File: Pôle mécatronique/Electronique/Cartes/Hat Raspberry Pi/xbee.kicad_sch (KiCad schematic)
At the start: 1 part

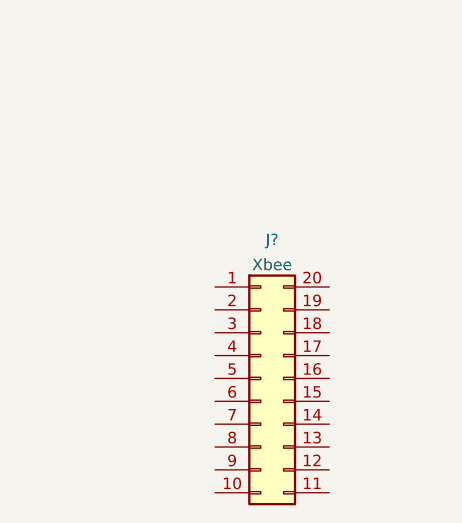
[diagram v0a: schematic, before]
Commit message: Reprise backup
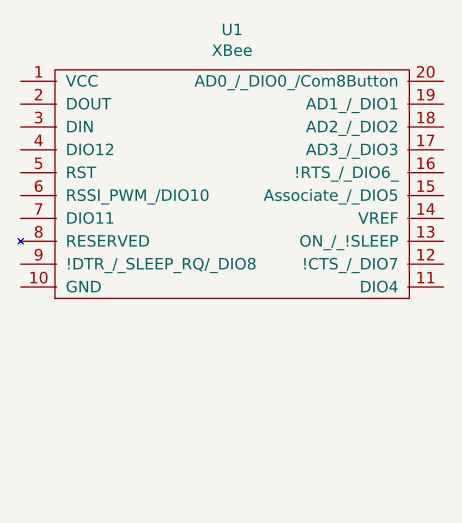
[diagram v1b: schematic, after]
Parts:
- removed J?: Xbee, symbol Connector_Generic:Conn_02x10_Counter_Clockwise
- added U1: XBee, Connecteurs:XBEE_PRO-20_THT, symbol bus_raspi-rescue:XBeePro-xbeepro
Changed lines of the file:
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@@
 (kicad_sch (version 20211123) (generator eeschema)
   (paper "A4")
-  (symbol (lib_id "Connector_Generic:Conn_02x10_Counter_Clockwise") (at 120.65 88.9 0) (unit 1)
-    (in_bom yes) (on_board yes) (fields_autoplaced)
-    (property "Reference" "J?" (id 0) (at 121.92 73.5035 0))
-    (property "Value" "Xbee" (id 1) (at 121.92 76.2786 0))
-    (property "Footprint" "" (id 2) (at 120.65 88.9 0)
+  (symbol (lib_id "bus_raspi-rescue:XBeePro-xbeepro") (at 93.98 85.09 0) (unit 1)
+    (in_bom yes) (on_board yes)
+    (property "Reference" "U1" (id 0) (at 117.475 50.165 0))
+    (property "Value" "XBee" (id 1) (at 117.475 52.4764 0))
+    (property "Footprint" "Connecteurs:XBEE_PRO-20_THT" (id 2) (at 85.09 72.39 0)
       (effects (font (size 1.27 1.27)) hide)
     )
-    (property "Datasheet" "~" (id 3) (at 120.65 88.9 0)
+    (property "Datasheet" "" (id 3) (at 85.09 72.39 0)
       (effects (font (size 1.27 1.27)) hide)
     )

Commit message: Revert "Update"
This reverts commit 5fda5d97c123c8007ff4d0ab26b634aa447f3b27.
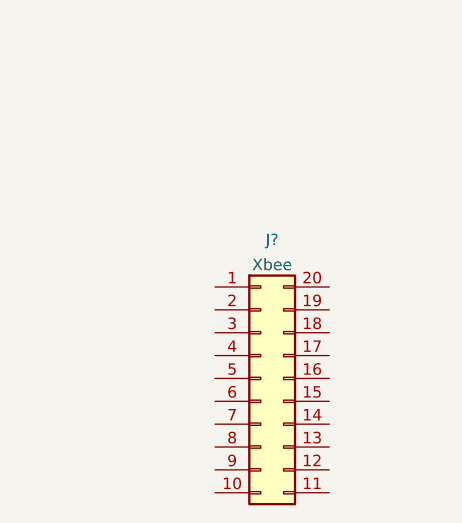
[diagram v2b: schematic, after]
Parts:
- removed U1: XBee, Connecteurs:XBEE_PRO-20_THT, symbol bus_raspi-rescue:XBeePro-xbeepro
- added J?: Xbee, symbol Connector_Generic:Conn_02x10_Counter_Clockwise
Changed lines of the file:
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@@
 (kicad_sch (version 20211123) (generator eeschema)
   (paper "A4")
-  (symbol (lib_id "bus_raspi-rescue:XBeePro-xbeepro") (at 93.98 85.09 0) (unit 1)
-    (in_bom yes) (on_board yes)
-    (property "Reference" "U1" (id 0) (at 117.475 50.165 0))
-    (property "Value" "XBee" (id 1) (at 117.475 52.4764 0))
-    (property "Footprint" "Connecteurs:XBEE_PRO-20_THT" (id 2) (at 85.09 72.39 0)
+  (symbol (lib_id "Connector_Generic:Conn_02x10_Counter_Clockwise") (at 120.65 88.9 0) (unit 1)
+    (in_bom yes) (on_board yes) (fields_autoplaced)
+    (property "Reference" "J?" (id 0) (at 121.92 73.5035 0))
+    (property "Value" "Xbee" (id 1) (at 121.92 76.2786 0))
+    (property "Footprint" "" (id 2) (at 120.65 88.9 0)
       (effects (font (size 1.27 1.27)) hide)
     )
-    (property "Datasheet" "" (id 3) (at 85.09 72.39 0)
+    (property "Datasheet" "~" (id 3) (at 120.65 88.9 0)
       (effects (font (size 1.27 1.27)) hide)
     )
